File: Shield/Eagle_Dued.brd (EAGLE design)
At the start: 177.8 x 104.1 mm, 76 parts, among them IC1 7805TV, IC2 LM340MP-05

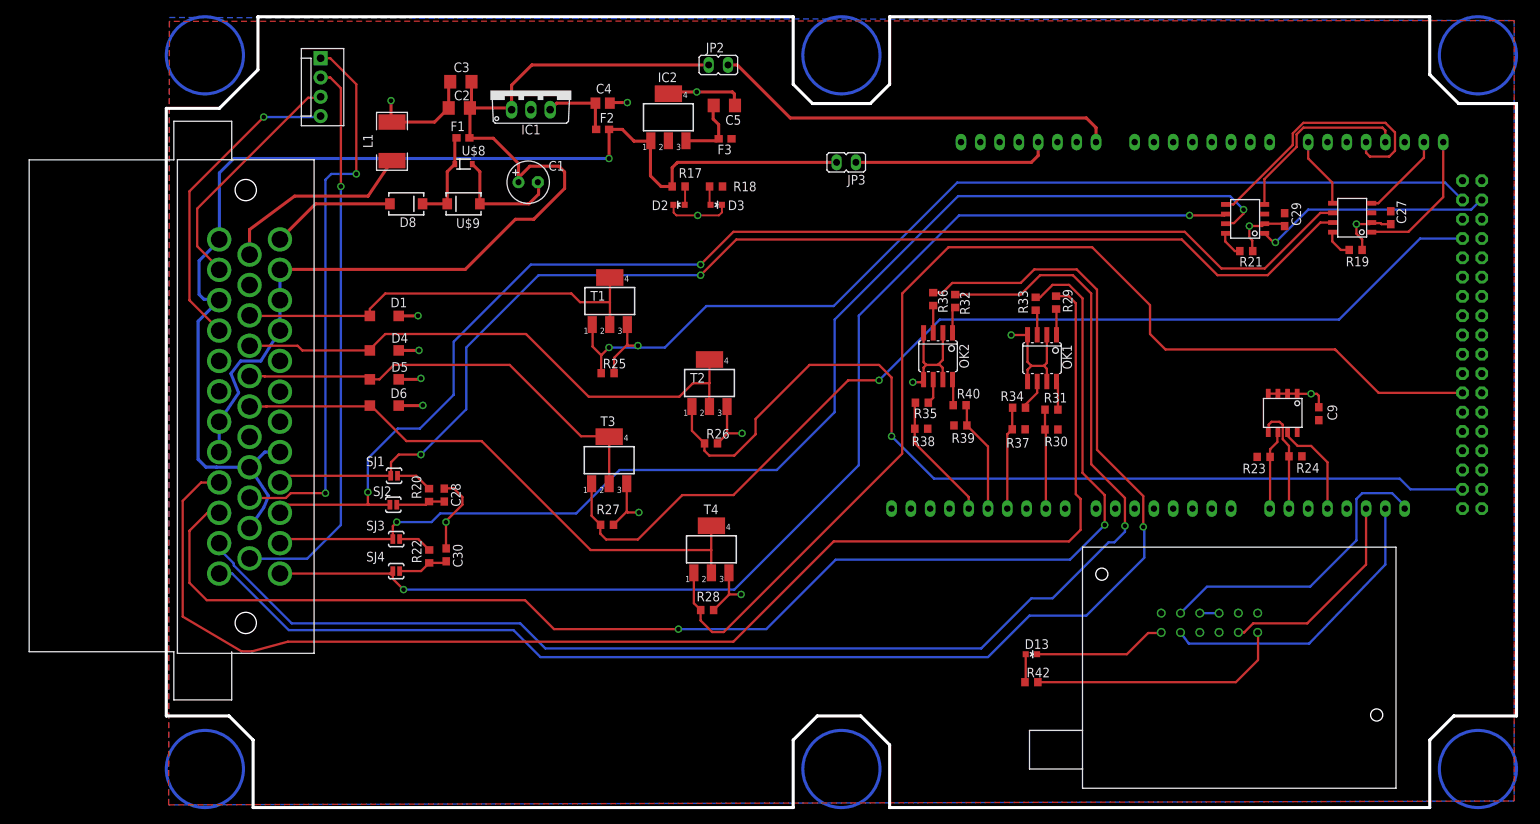
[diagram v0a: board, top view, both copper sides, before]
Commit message: Continued finagling with the dued board.
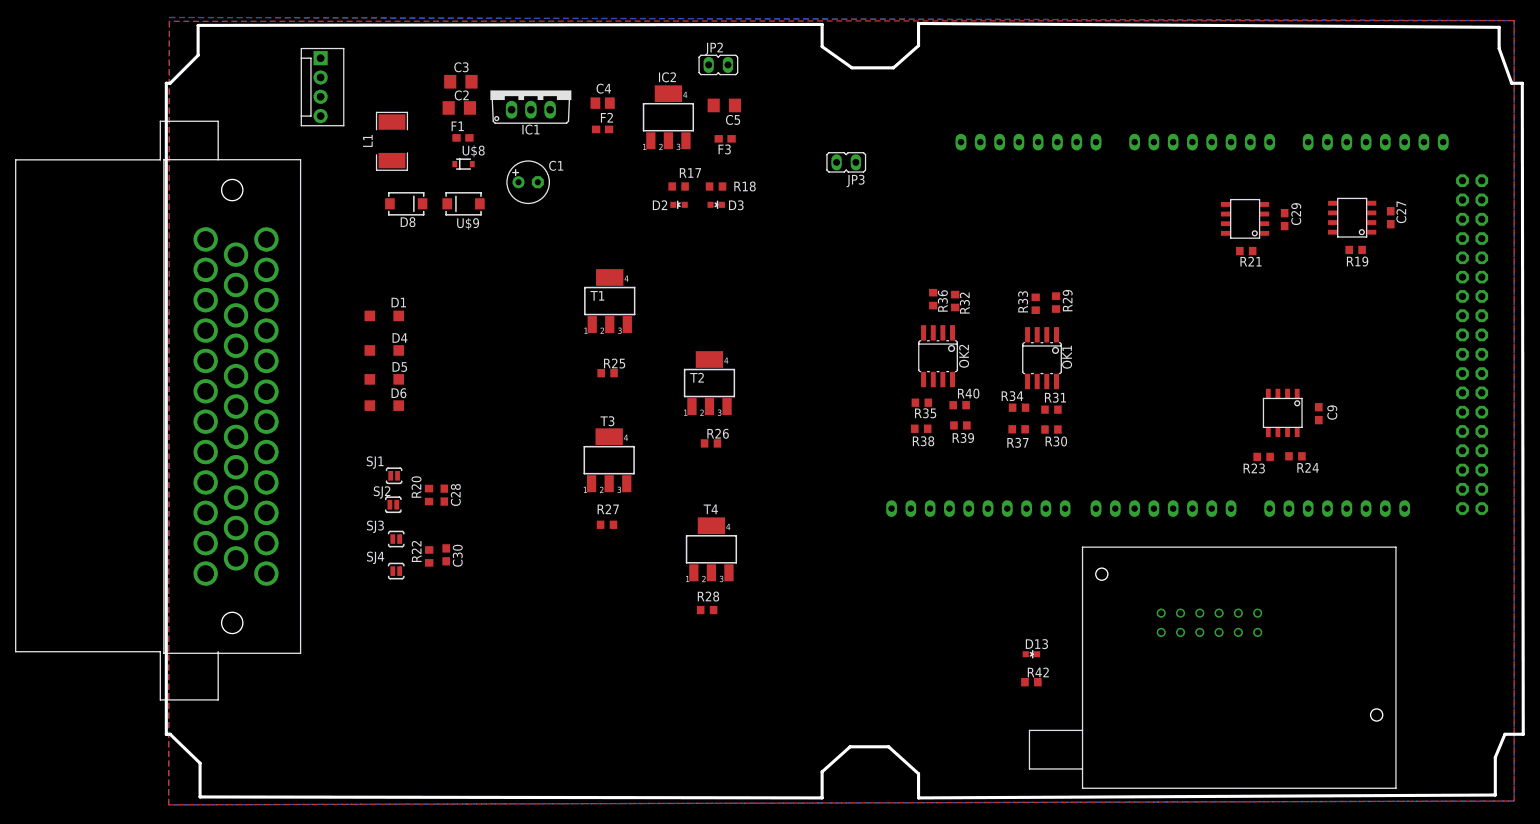
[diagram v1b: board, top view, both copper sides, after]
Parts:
- moved U$3 1.78 mm to (13.2, 54.8)
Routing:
- net DIN4: track 193.6 -> 0.00 mm, vias 1 -> 0
- net DIN3: track 185.1 -> 0.00 mm, vias 1 -> 0
- net GND: track 180.5 -> 0.00 mm, vias 18 -> 0
- net DIN1: track 179.9 -> 0.00 mm
- net DIN2: track 179.1 -> 0.00 mm, vias 2 -> 0
- net CANL0: track 169.6 -> 0.00 mm, vias 2 -> 0
- net CANH0: track 162.5 -> 0.00 mm, vias 2 -> 0
- net CANL1: track 158.3 -> 0.00 mm, vias 2 -> 0
- net +5V: track 158.2 -> 0.00 mm, vias 1 -> 0
- net CANH1: track 158.1 -> 0.00 mm, vias 2 -> 0
- net DIGOUT4: track 151.1 -> 0.00 mm
- net DIGOUT3: track 137.4 -> 0.00 mm, vias 1 -> 0
- net +12V: track 134.2 -> 0.00 mm
- net DIGOUT1: track 130.7 -> 0.00 mm, vias 1 -> 0
- net DIGOUT2: track 124.1 -> 0.00 mm, vias 1 -> 0
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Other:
- board size 177.8 x 104.1 mm -> 178.7 x 102 mm
